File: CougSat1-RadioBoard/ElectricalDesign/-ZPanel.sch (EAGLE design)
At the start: 44 parts, among them J1 High Gain Antenna, J2 Deployables, J3 High Gain +, J4 ADCS, J5 Flap +X, J6 Flap -X, J7 Flap +Y, J8 Flap -Y, U1 AD7291, U3 AD8515

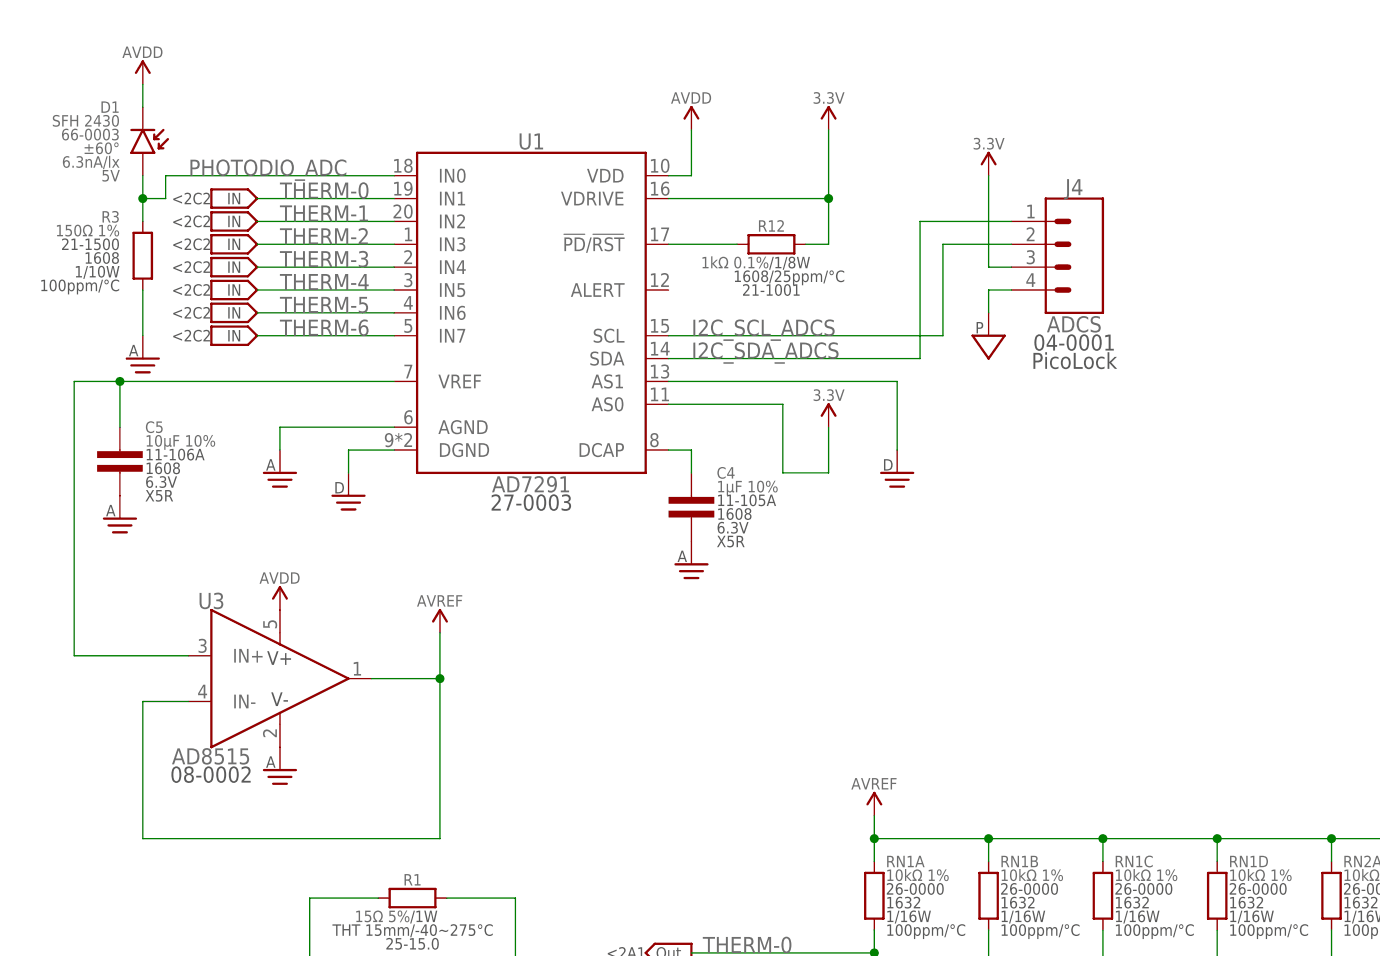
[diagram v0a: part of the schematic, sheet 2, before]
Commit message: Ready For Review
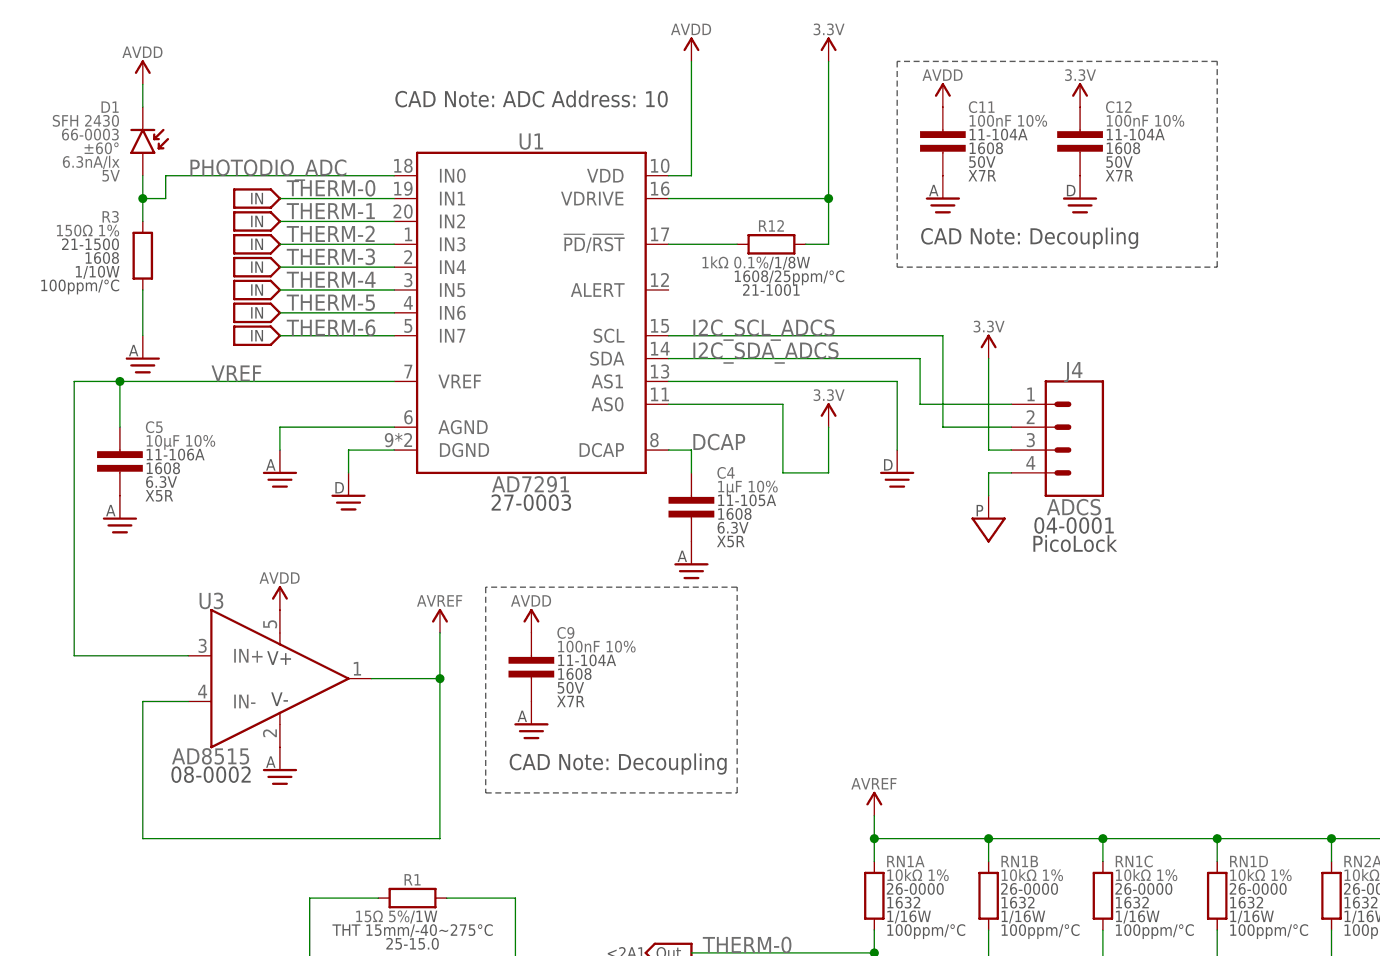
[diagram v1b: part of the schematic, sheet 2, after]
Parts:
- added C11, C12, C9: 100nF 10%, CougsInSpace-Capacitors:CAP-V-100NF-1608
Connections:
- net N$6 renamed PD/RST
- net N$8 renamed DCAP
- net N$9 renamed VREF
- net 3.3V: now also C12.1
- net AGND: now also C11.2, C9.2
- net AVDD: now also C11.1, C9.1
- net DGND: now also C12.2
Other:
- note added: "96mm"
- note added: "CAD Note: ADC Address: 10"
- note added: "CAD Note: Center Point"
- note added: "CAD Note: Decoupling"
- note removed: "<2C2"
- moved on the sheet: J4

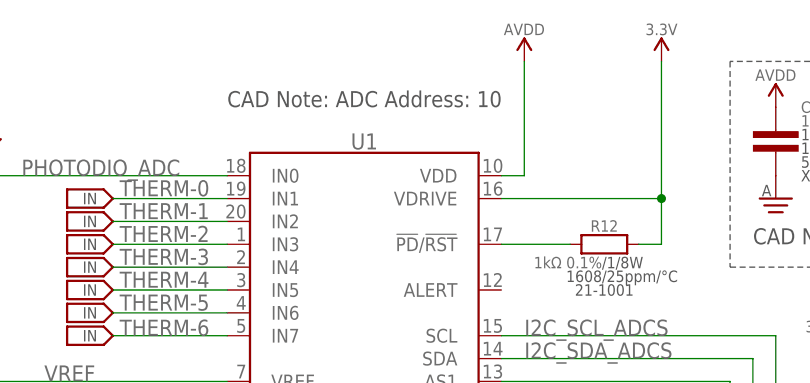
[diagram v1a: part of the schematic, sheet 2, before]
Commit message: 1.0.3
Ready for review
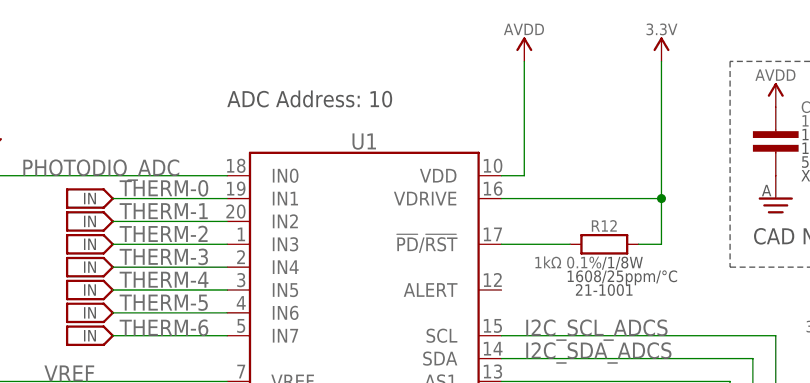
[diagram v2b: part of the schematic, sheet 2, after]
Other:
- note added: "ADC Address: 10"
- note removed: "CAD Note: ADC Address: 10"
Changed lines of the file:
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@@
 <setting verticaltext="up"/>
 </settings>
-<grid distance="1" unitdist="mm" unit="mm" style="lines" multiple="1" display="yes" altdistance="1" altunitdist="mm" altunit="mm"/>
+<grid distance="0.1" unitdist="inch" unit="inch" style="lines" multiple="1" display="no" altdistance="0.01" altunitdist="inch" altunit="inch"/>
 <layers>
 <layer number="1" name="Top" color="4" fill="1" visible="no" active="no"/>
@@
 <wire x1="78.74" y1="106.68" x2="78.74" y2="129.54" width="0.1524" layer="97" style="shortdash"/>
 <wire x1="78.74" y1="129.54" x2="50.8" y2="129.54" width="0.1524" layer="97" style="shortdash"/>
-<text x="40.64" y="182.88" size="1.778" layer="97">CAD Note: ADC Address: 10</text>
+<text x="40.64" y="182.88" size="1.778" layer="97">ADC Address: 10</text>
 </plain>
 <instances>
